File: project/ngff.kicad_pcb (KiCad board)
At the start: 4 copper layers, 90 x 40 mm, 62 parts, among them J1 KUSBX-BS1N9-1-BL30, J2 2199119-3, J3 Jack-DC, J4 SIM8060-6-1-14-00-A, J5 Conn_01x03_Male, J6 SIM8060-6-1-14-00-A, SW1 KMR221GLFS, U1 AP62301WU7

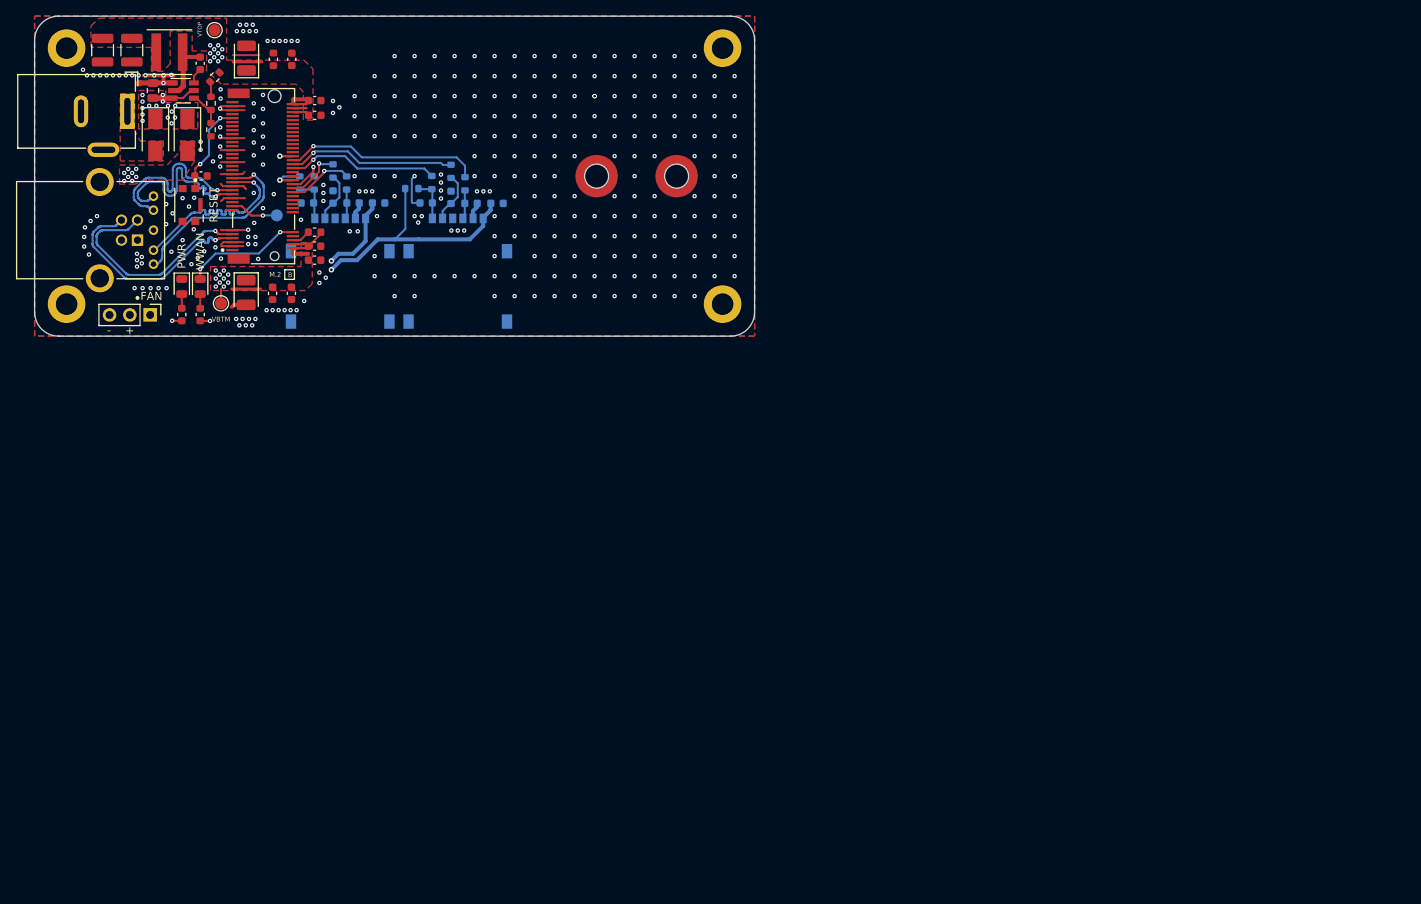
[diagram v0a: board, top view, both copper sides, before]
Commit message: update
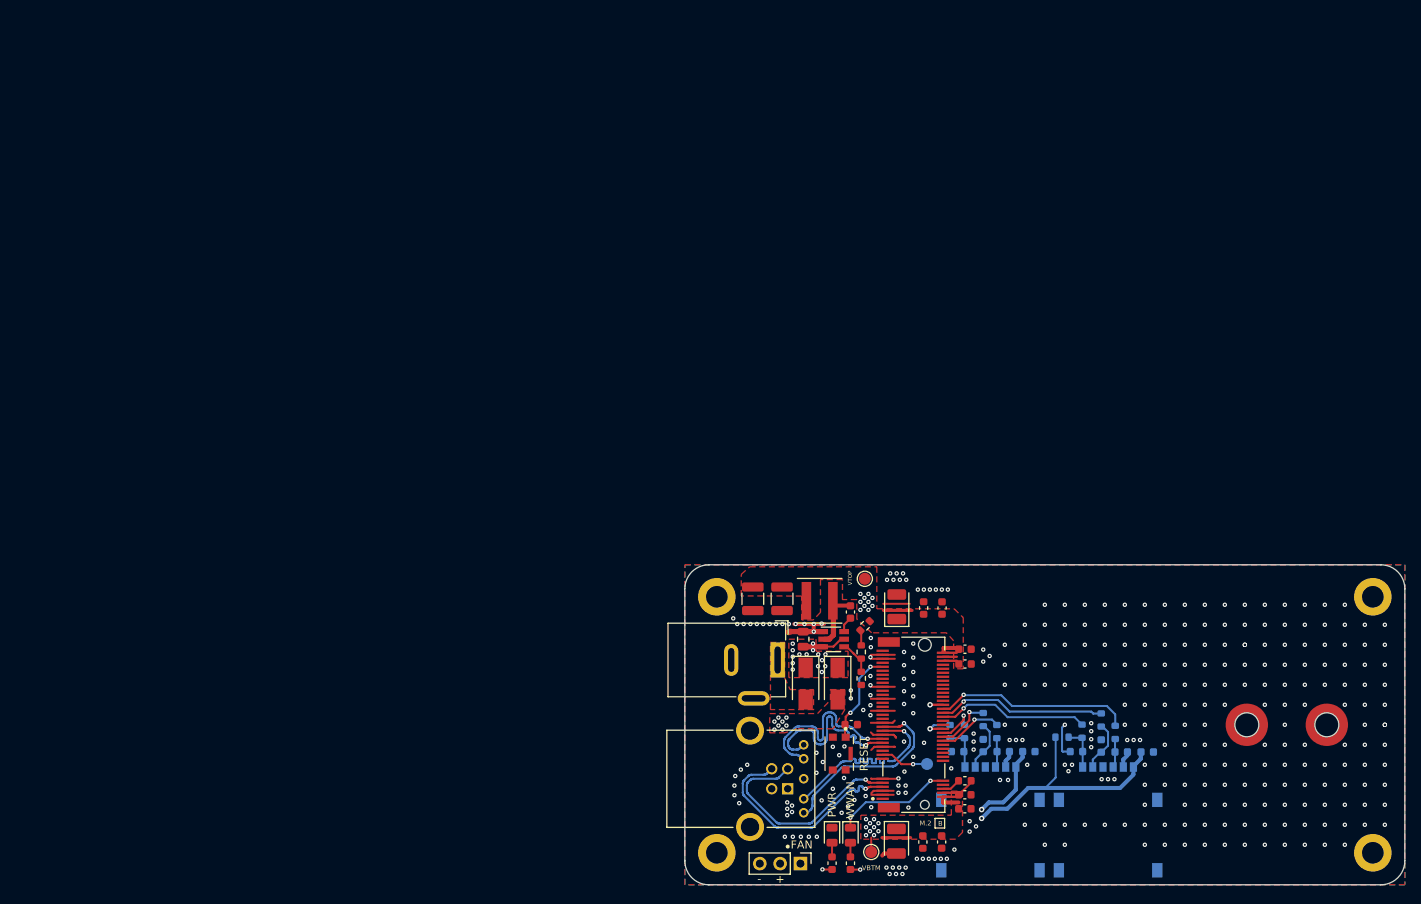
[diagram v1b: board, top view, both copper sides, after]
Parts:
- removed the REF** at (4.00, 36.0)
- removed the REF** at (86.0, 36.0)
- removed the REF** at (86.0, 4.00)
- added REF**: MountingHole_2.7mm_M2.5_DIN965_Pad, MountingHole:MountingHole_2.7mm_M2.5_DIN965_Pad, F.Cu at (85.3, 104.6)
- added REF**: MountingHole_2.7mm_M2.5_DIN965_Pad, MountingHole:MountingHole_2.7mm_M2.5_DIN965_Pad, F.Cu at (167.3, 104.6)
- added REF**: MountingHole_2.7mm_M2.5_DIN965_Pad, MountingHole:MountingHole_2.7mm_M2.5_DIN965_Pad, F.Cu at (167.3, 72.6)
- moved C10 106.3 mm to (111.0, 103.2)
- moved C11 106.3 mm to (113.4, 103.2)
- moved C14 106.3 mm to (102.1, 88.6)
- moved C16 106.3 mm to (139.1, 92.0)
- moved C17 106.3 mm to (135.8, 92.0)
- moved C18 106.3 mm to (133.3, 91.2)
- moved C20 106.3 mm to (124.3, 91.9)
- moved C21 106.3 mm to (121.1, 91.9)
- moved C22 106.3 mm to (118.6, 91.2)
- moved C23 106.3 mm to (115.4, 91.9)
- moved D1 106.3 mm to (100.4, 83.4)
- moved D2 106.3 mm to (96.4, 83.4)
- moved J5 106.3 mm to (95.7, 105.9)
- moved R10 106.3 mm to (120.3, 89.4)
- moved R11 106.3 mm to (118.6, 87.9)
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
